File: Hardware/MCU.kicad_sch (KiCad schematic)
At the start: 38 parts, among them J3 SWD/ExtTrig, J4 EXT_GPIOS, SW2 SW_MCU_NRST, U3 STM32F411CEUx, Y1 16MHz

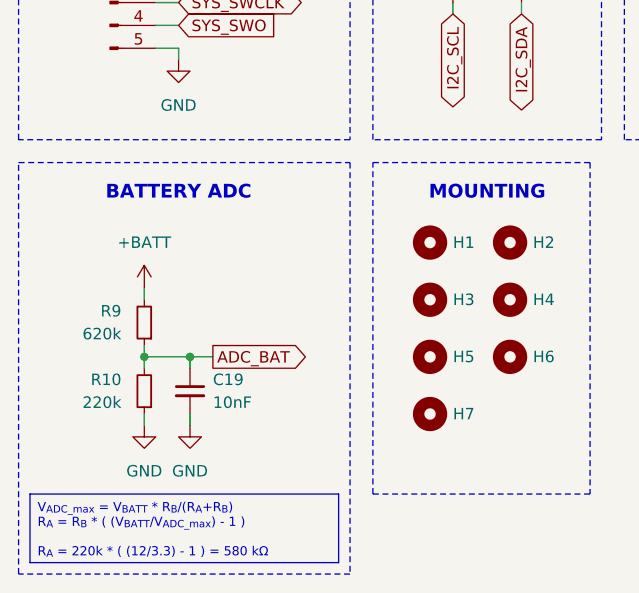
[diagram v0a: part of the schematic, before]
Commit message: Developing HW - routing
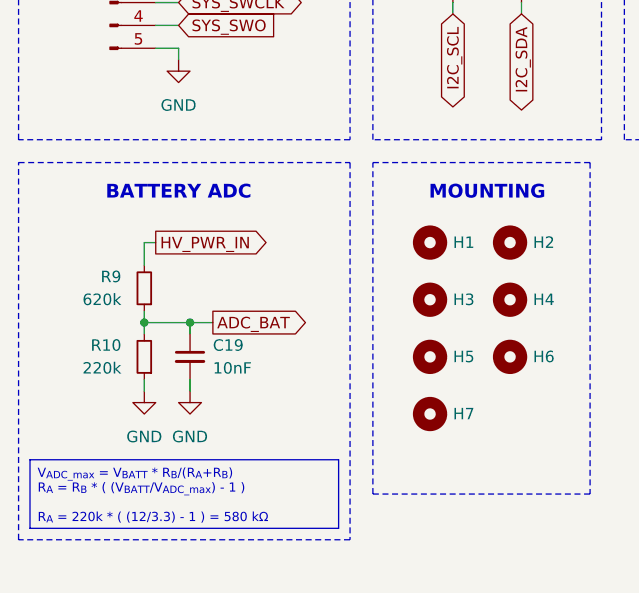
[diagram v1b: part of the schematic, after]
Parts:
- JP3, JP4: footprint Jumper:SolderJumper-3_P1.3mm_Open_RoundedPad1.0x1.5mm -> BRS_Footprints:SMD_SolderJumper_Triple_Small
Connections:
- net +BATT renamed HV_PWR_IN
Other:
- moved on the sheet: C19, R10, R9

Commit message: Working on power source
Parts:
- C11, C16, C17, C18, C19, C6: footprint Capacitor_SMD:C_0603_1608Metric -> Capacitor_SMD:C_0402_1005Metric
- JP3, JP4: footprint BRS_Footprints:SMD_SolderJumper_Triple_Small -> BRS_Footprints:SMD_SolderJumper_Triple_Micro
- R10, R2, R4, R5, R6, R9: footprint Resistor_SMD:R_0603_1608Metric -> Resistor_SMD:R_0402_1005Metric
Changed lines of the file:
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@@
 			)
 		)
-		(property "Footprint" "Resistor_SMD:R_0603_1608Metric"
+		(property "Footprint" "Resistor_SMD:R_0402_1005Metric"
 			(at 110.49 153.67 0)
 			(effects
@@
 			)
 		)
-		(property "Footprint" "Capacitor_SMD:C_0603_1608Metric"
+		(property "Footprint" "Capacitor_SMD:C_0402_1005Metric"
 			(at 105.41 158.75 0)
 			(effects
@@
 			)
 		)
-		(property "Footprint" "Resistor_SMD:R_0603_1608Metric"
+		(property "Footprint" "Resistor_SMD:R_0402_1005Metric"
 			(at 110.49 110.49 0)
 			(effects
@@
 			)
 		)
-		(property "Footprint" "Capacitor_SMD:C_0603_1608Metric"
+		(property "Footprint" "Capacitor_SMD:C_0402_1005Metric"
 			(at 104.14 54.61 0)
 			(effects
@@
 			)
 		)
-		(property "Footprint" "BRS_Footprints:SMD_SolderJumper_Triple_Small"
+		(property "Footprint" "BRS_Footprints:SMD_SolderJumper_Triple_Micro"
 			(at 125.73 153.67 0)
 			(effects
@@
 			)
 		)
-		(property "Footprint" "BRS_Footprints:SMD_SolderJumper_Triple_Small"
+		(property "Footprint" "BRS_Footprints:SMD_SolderJumper_Triple_Micro"
 			(at 176.53 153.67 0)
 			(effects
@@
 			)
 		)
-		(property "Footprint" "Resistor_SMD:R_0603_1608Metric"
+		(property "Footprint" "Resistor_SMD:R_0402_1005Metric"
 			(at 99.06 232.41 0)
 			(effects
@@
 			)
 		)
-		(property "Footprint" "Capacitor_SMD:C_0603_1608Metric"
+		(property "Footprint" "Capacitor_SMD:C_0402_1005Metric"
 			(at 110.49 120.65 0)
 			(effects
@@
 			)
 		)
-		(property "Footprint" "Capacitor_SMD:C_0603_1608Metric"
+		(property "Footprint" "Capacitor_SMD:C_0402_1005Metric"
 			(at 156.21 158.75 0)
 			(effects
@@
 			)
 		)
-		(property "Footprint" "Resistor_SMD:R_0603_1608Metric"
+		(property "Footprint" "Resistor_SMD:R_0402_1005Metric"
 			(at 99.06 224.79 0)
 			(effects
@@
 			)
 		)
-		(property "Footprint" "Capacitor_SMD:C_0603_1608Metric"
+		(property "Footprint" "Capacitor_SMD:C_0402_1005Metric"
 			(at 160.02 81.28 0)
 			(effects
@@
 			)
 		)
-		(property "Footprint" "Resistor_SMD:R_0603_1608Metric"
+		(property "Footprint" "Resistor_SMD:R_0402_1005Metric"
 			(at 161.29 153.67 0)
 			(effects
@@
 			)
 		)
-		(property "Footprint" "Resistor_SMD:R_0603_1608Metric"
+		(property "Footprint" "Resistor_SMD:R_0402_1005Metric"
 			(at 105.41 116.84 0)
 			(effects
@@
 			)
 		)
-		(property "Footprint" "Capacitor_SMD:C_0603_1608Metric"
+		(property "Footprint" "Capacitor_SMD:C_0402_1005Metric"
 			(at 104.14 232.41 0)
 			(effects
